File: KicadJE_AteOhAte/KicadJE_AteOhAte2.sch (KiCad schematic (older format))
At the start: 72 parts, among them J201 In_1, J202 In 2, J203 Out 1, J204 Out 2, J205 Out Final, P201 Doepfer_Power_10pin, SW201 Out 1, SW202 In or cascade, SW203 Out 2 FB, SW204 In or cascade, SW205 HI/LO, U201 TL072, U202 TL072

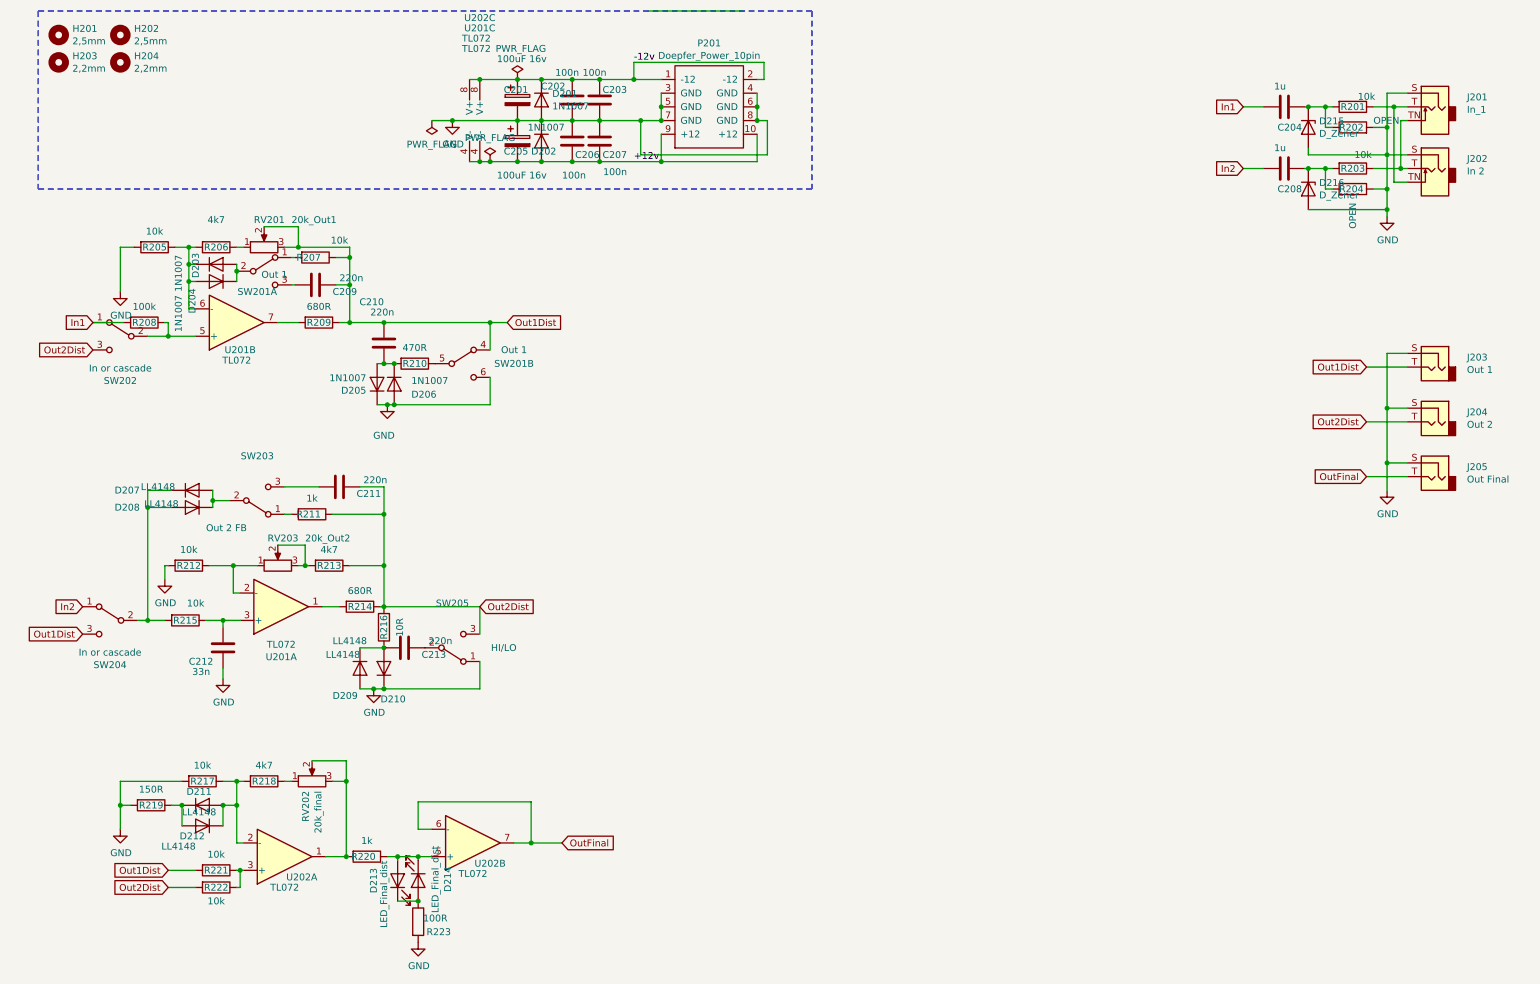
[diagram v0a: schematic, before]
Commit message: Sch initiating
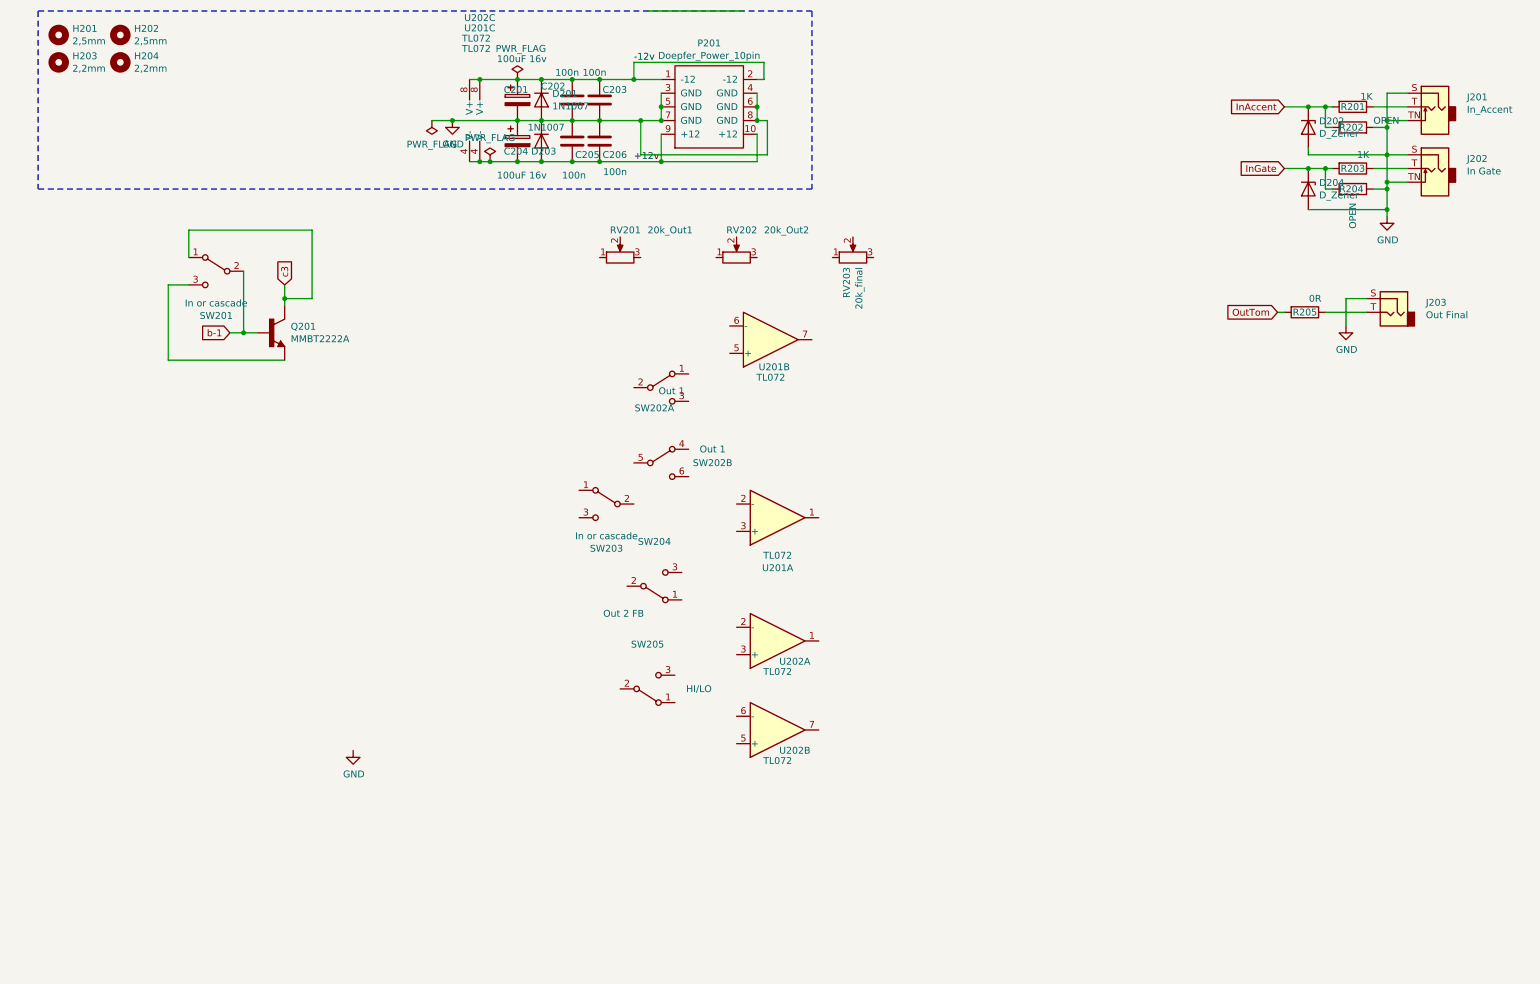
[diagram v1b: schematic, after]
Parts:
- removed C204, C208: 1u, Capacitor_SMD:C_0805_2012Metric_Pad1.15x1.40mm_HandSolder, symbol Device:C
- removed C209, C210, C211, C213: 220n, Capacitor_SMD:C_0805_2012Metric_Pad1.15x1.40mm_HandSolder, symbol Device:C
- removed C212: 33n, Capacitor_SMD:C_0805_2012Metric_Pad1.15x1.40mm_HandSolder, symbol Device:C
- removed D203, D204, D205, D206: 1N1007, Diode_SMD:D_SOD-123, symbol Device:D
- removed D207, D208, D209, D210, D211, D212: LL4148, Diode_SMD:D_MiniMELF, symbol Diode:LL4148
- removed D213, D214: LED_Final_dist, LED_THT:LED_D3.0mm, symbol Device:LED
- removed J203: Out 1, AJ-Dropbox-Kicad:PJ301SM, symbol Connector:AudioJack2
- removed J204: Out 2, AJ-Dropbox-Kicad:PJ301SM, symbol Connector:AudioJack2
- removed R206, R213, R218: 4k7, Resistor_SMD:R_0805_2012Metric_Pad1.15x1.40mm_HandSolder, symbol Device:R
- removed R207, R212, R215, R217, R221, R222: 10k, Resistor_SMD:R_0805_2012Metric_Pad1.15x1.40mm_HandSolder, symbol Device:R
- removed R208: 100k, Resistor_SMD:R_0805_2012Metric_Pad1.15x1.40mm_HandSolder, symbol Device:R
- removed R209, R214: 680R, Resistor_SMD:R_0805_2012Metric_Pad1.15x1.40mm_HandSolder, symbol Device:R
- removed R210: 470R, Resistor_SMD:R_0805_2012Metric_Pad1.15x1.40mm_HandSolder, symbol Device:R
- removed R211, R220: 1k, Resistor_SMD:R_0805_2012Metric_Pad1.15x1.40mm_HandSolder, symbol Device:R
- removed R216: 10R, Resistor_SMD:R_0805_2012Metric_Pad1.15x1.40mm_HandSolder, symbol Device:R
- removed R219: 150R, Resistor_SMD:R_0805_2012Metric_Pad1.15x1.40mm_HandSolder, symbol Device:R
- removed R223: 100R, Resistor_SMD:R_0805_2012Metric_Pad1.15x1.40mm_HandSolder, symbol Device:R
- added Q201: MMBT2222A, Package_TO_SOT_SMD:SOT-23_Handsoldering, symbol MMBT2222A:MMBT2222A
- J201: value In_1 -> In_Accent; footprint AJ-Dropbox-Kicad:PJ301SM -> Connector_Audio:Jack_3.5mm_Ledino_KB3SPRS_Horizontal
- J202: value In 2 -> In Gate; footprint AJ-Dropbox-Kicad:PJ301SM -> Connector_Audio:Jack_3.5mm_Ledino_KB3SPRS_Horizontal
- R201, R203: value 10k -> 1K
- R205: value 10k -> 0R
- renumbered C205 to C204, C206 to C205, C207 to C206, D215 to D202, D202 to D203, D216 to D204, J205 to J203, RV203 to RV202, RV202 to RV203, SW202 to SW201, SW201 to SW202, SW204 to SW203, SW203 to SW204
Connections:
- net labels added: InAccent, InGate, OutTom, b-1, c3
- net labels removed: In1, In2, Out1Dist, Out2Dist, OutFinal
- wire segments 196 -> 81
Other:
- moved on the sheet: J203, RV201, RV202, RV203, SW201, SW202A, SW202B, SW203, SW204, SW205, U201A, U201B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
